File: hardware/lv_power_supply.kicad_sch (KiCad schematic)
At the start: 13 parts, among them IC1 L7812ABV, Q1 PMOS, Q2 PMOS

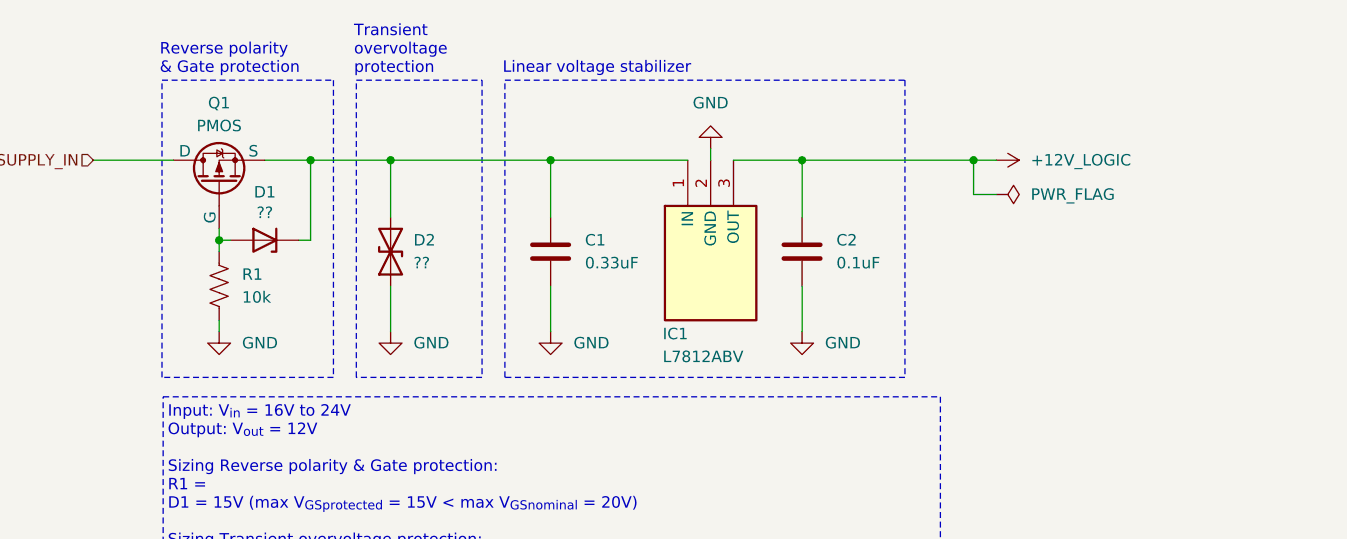
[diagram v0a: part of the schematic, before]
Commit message: fix ERC power line errors
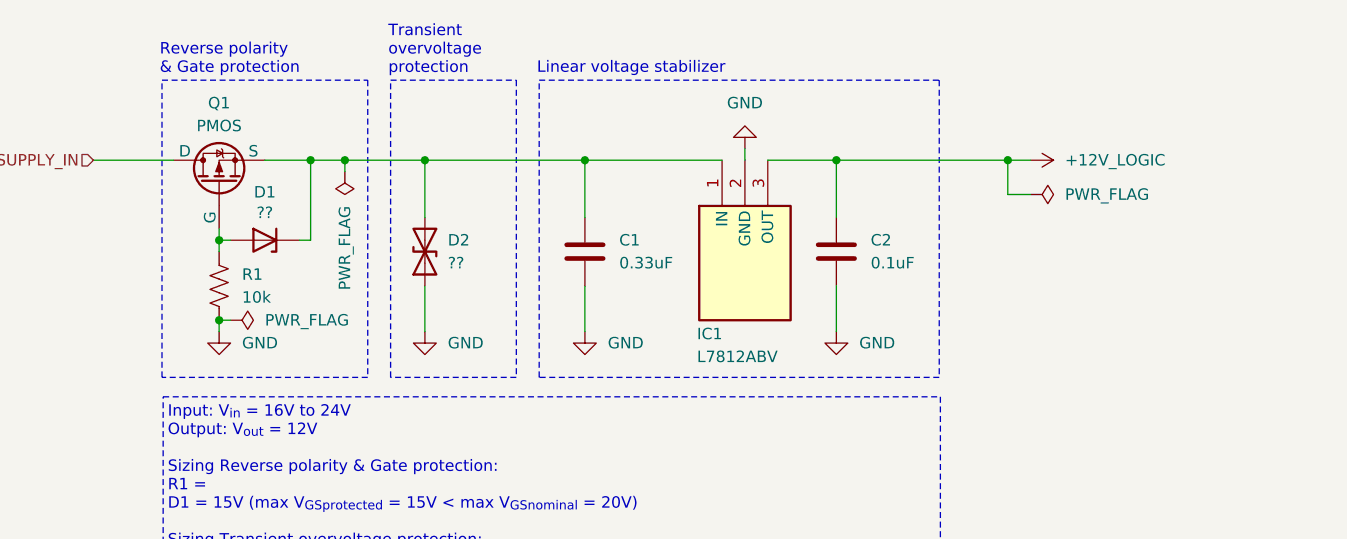
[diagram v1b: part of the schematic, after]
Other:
- moved on the sheet: C1, C2, D2, IC1

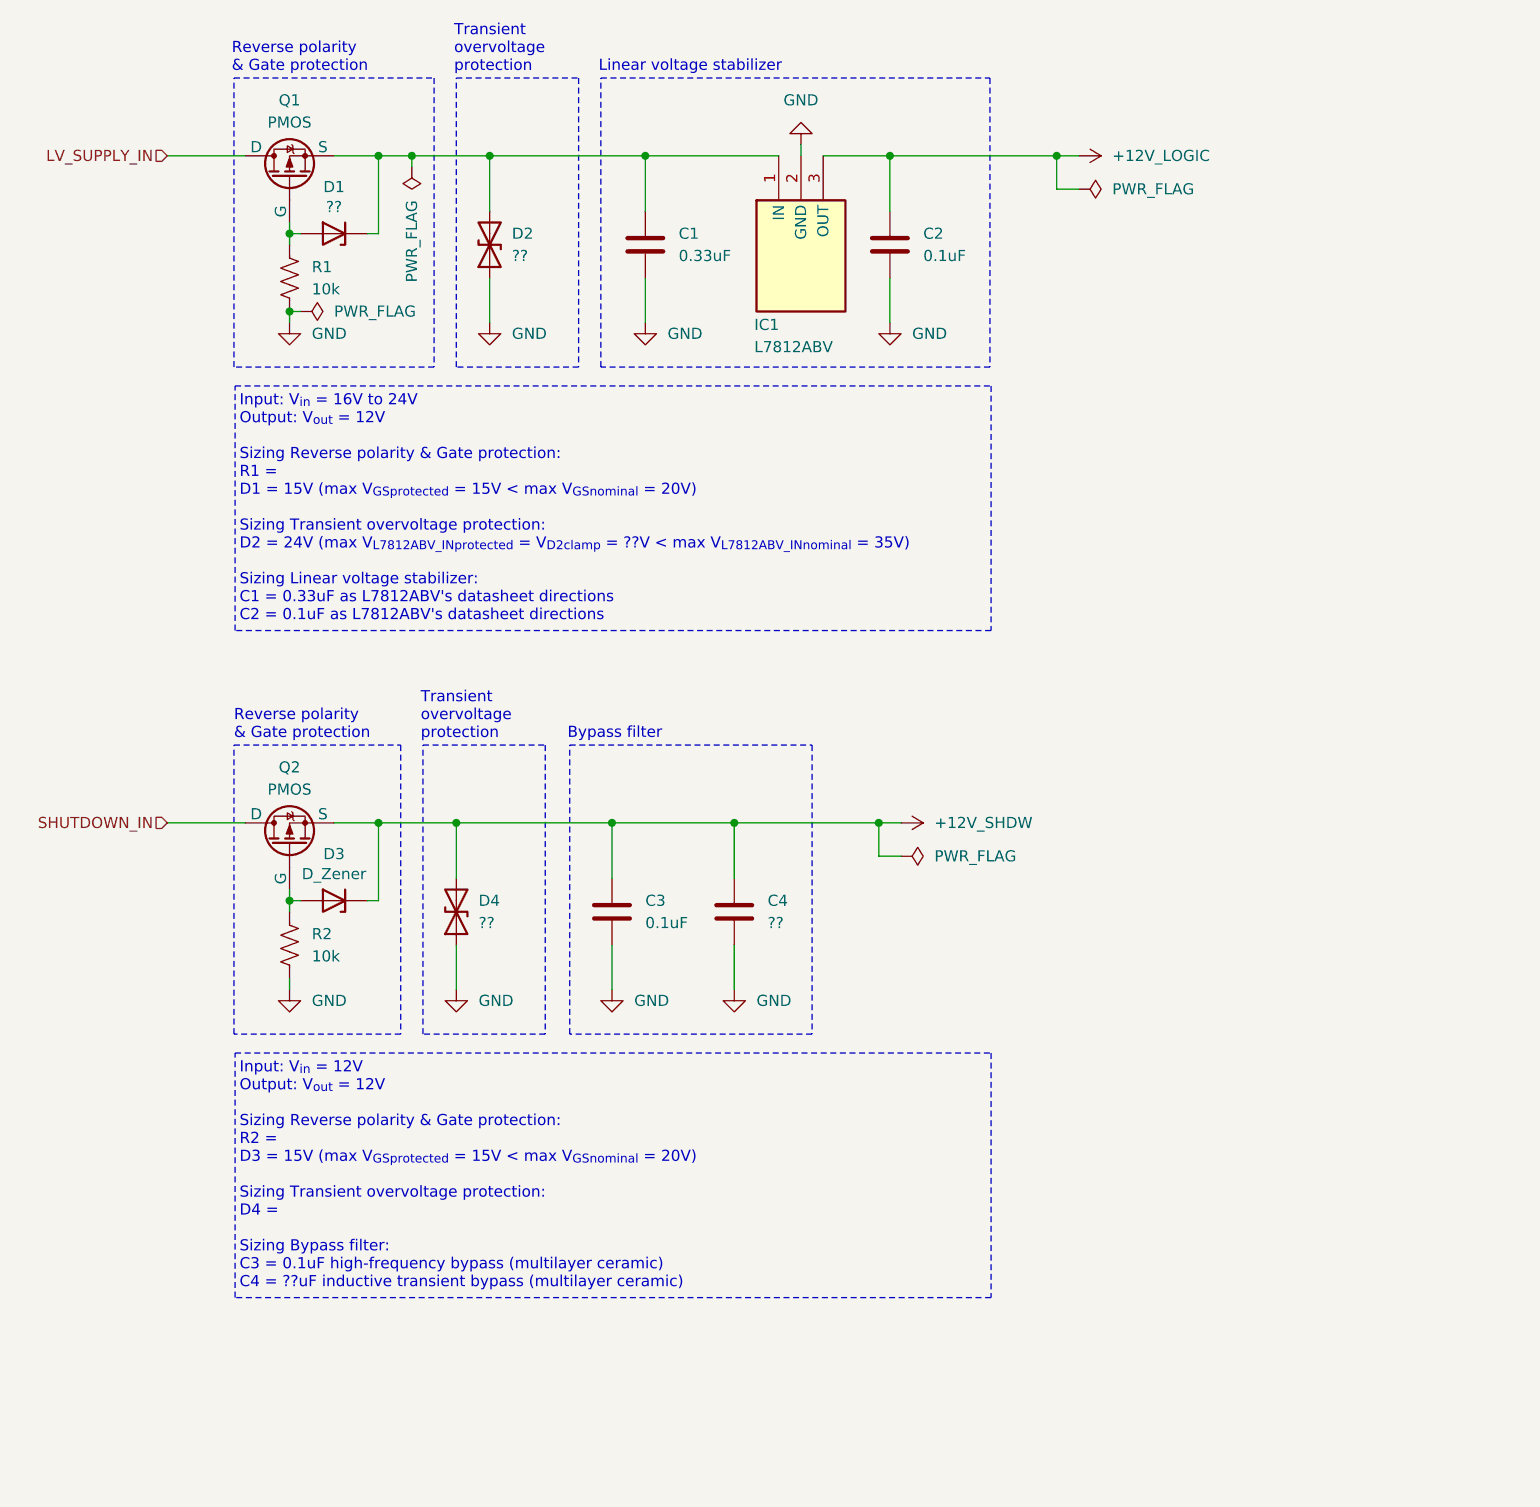
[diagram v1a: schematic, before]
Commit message: start power supply and logic sizing
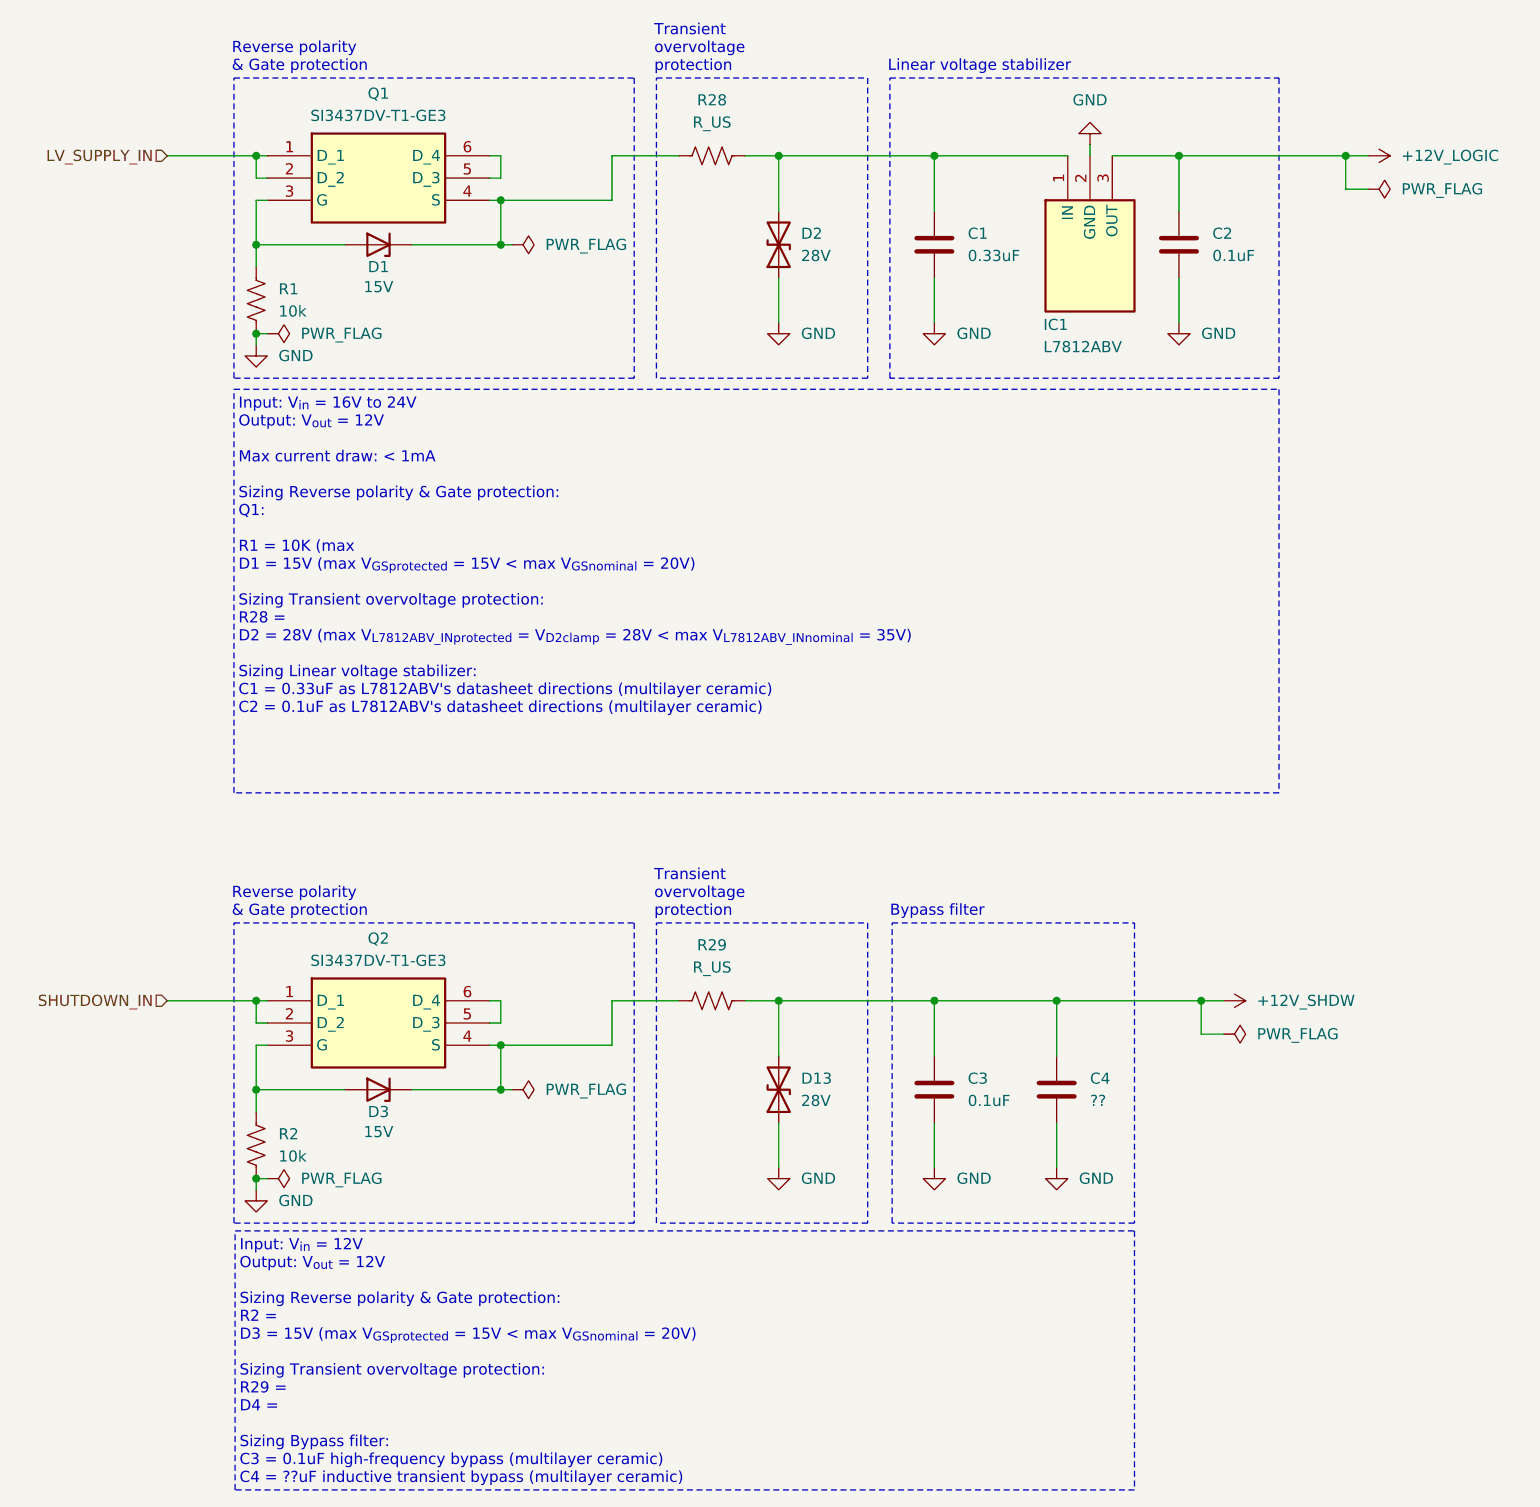
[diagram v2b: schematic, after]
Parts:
- removed D4: ??, symbol Device:D_TVS
- removed Q1, Q2: PMOS, symbol Simulation_SPICE:PMOS
- added D13: 28V, symbol Device:D_TVS
- added Q1, Q2: SI3437DV-T1-GE3, SOT95P284X110-6N, symbol Libary_Loader:SI3437DV-T1-GE3
- added R28, R29: R_US, symbol Device:R_US
- D1: value ?? -> 15V
- D2: value ?? -> 28V
- D3: value D_Zener -> 15V
- IC1: footprint TO255P460X1020X2008-3P -> Library_Loader:TO255P460X1020X2008-3P
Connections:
- net +12V_SHDW: now also D13.2 (A2), R29.2; no longer D3.1 (K)
- net GND: now also D13.1 (A1)
- net LV_SUPPLY_IN: now also Q1.1 (D_1), Q1.2 (D_2)
- net SHUTDOWN_IN: now also Q2.1 (D_1), Q2.2 (D_2)
- net at D3.2 (A), R2.1: now also Q2.3 (G)
- net at C1.1, D2.2 (A2), IC1.1 (IN): now also R28.2; no longer D1.1 (K)
- net at D1.2 (A), R1.1: now also Q1.3 (G)
- new net: D1.1 (K), Q1.4 (S), R28.1
- new net: Q1.5 (D_3), Q1.6 (D_4)
- new net: D3.1 (K), Q2.4 (S), R29.1
- new net: Q2.5 (D_3), Q2.6 (D_4)
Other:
- note added: "Input: V_{in} = 12V Output: V_{out} = 12V Sizing Reverse polarity & Gate protection: R2 = D3 = 15V (max V_{GS}_{protected} = 15V < max V_{GS}_{nominal} = 20V) Sizing Transient overvoltage protection: R29 = D4 = Sizing Bypass filter: C3 = 0.1uF high-frequency bypass (multilayer ceramic) C4 = ??uF inductive transient bypass (multilayer ceramic)"
- note added: "Input: V_{in} = 16V to 24V Output: V_{out} = 12V Max current draw: < 1mA Sizing Reverse polarity & Gate protection: Q1: R1 = 10K (max D1 = 15V (max V_{GS}_{protected} = 15V < max V_{GS}_{nominal} = 20V) Sizing Transient overvoltage protection: R28 = D2 = 28V (max V_{L7812ABV_IN}_{protected} = V_{D2}_{clamp} = 28V < max V_{L7812ABV_IN}_{nominal} = 35V) Sizing Linear voltage stabilizer: C1 = 0.33uF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"
- note removed: "Input: V_{in} = 12V Output: V_{out} = 12V Sizing Reverse polarity & Gate protection: R2 = D3 = 15V (max V_{GS}_{protected} = 15V < max V_{GS}_{nominal} = 20V) Sizing Transient overvoltage protection: D4 = Sizing Bypass filter: C3 = 0.1uF high-frequency bypass (multilayer ceramic) C4 = ??uF inductive transient bypass (multilayer ceramic)"
- note removed: "Input: V_{in} = 16V to 24V Output: V_{out} = 12V Sizing Reverse polarity & Gate protection: R1 = D1 = 15V (max V_{GS}_{protected} = 15V < max V_{GS}_{nominal} = 20V) Sizing Transient overvoltage protection: D2 = 24V (max V_{L7812ABV_IN}_{protected} = V_{D2}_{clamp} = ??V < max V_{L7812ABV_IN}_{nominal} = 35V) Sizing Linear voltage stabilizer: C1 = 0.33uF as L7812ABV's datasheet directions C2 = 0.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"
- moved on the sheet: C1, C2, C3, C4, D1, D2, IC1, R1
